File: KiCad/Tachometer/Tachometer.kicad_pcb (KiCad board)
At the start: 2 copper layers, 118.6 x 100 mm, 24 parts, among them J1 PJ301M-12, J2 Conn_01x15_MountingPin, J3 Conn_01x15_MountingPin, Q1 2N3904, Q2 2N3904

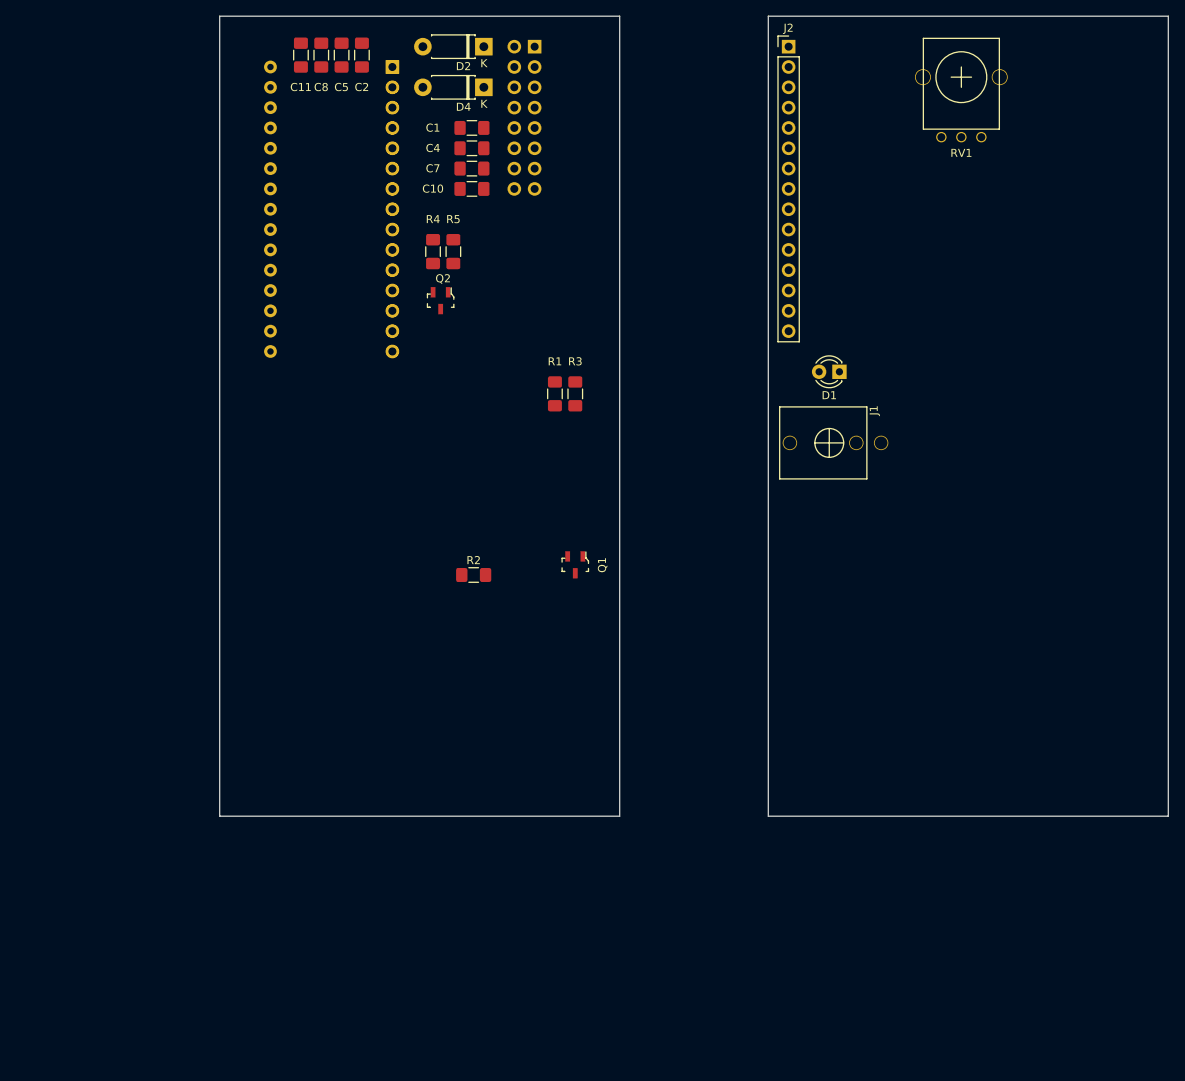
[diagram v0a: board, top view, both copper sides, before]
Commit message: ruffplaced pcb
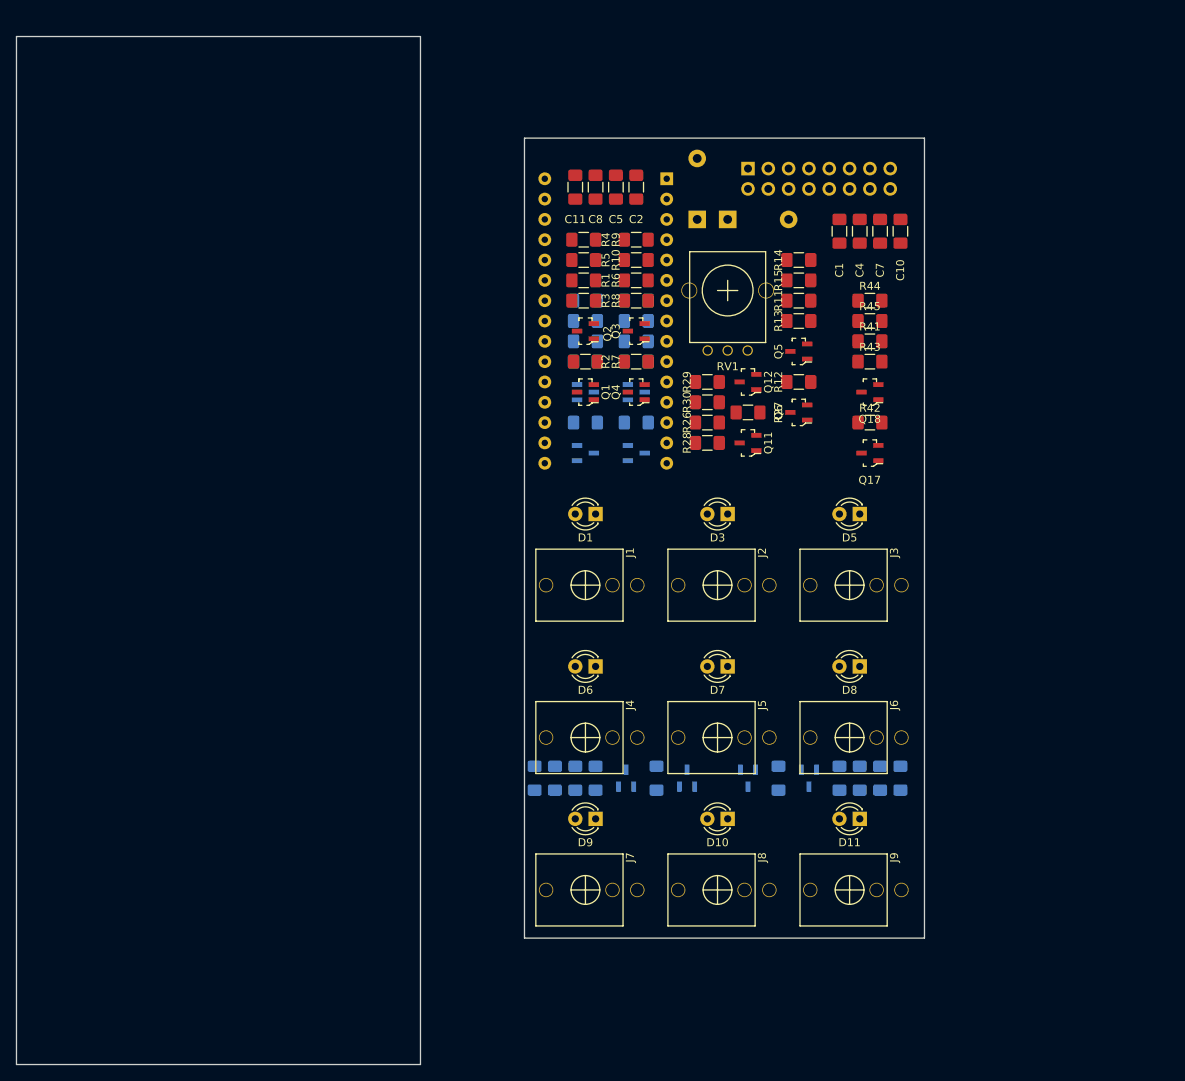
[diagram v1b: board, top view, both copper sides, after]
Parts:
- added D10: LED, LED_THT:LED_D3.0mm_FlatTop, F.Cu at (203.2, 123.2)
- added D11: LED, LED_THT:LED_D3.0mm_FlatTop, F.Cu at (219.7, 123.2)
- added D3: LED, LED_THT:LED_D3.0mm_FlatTop, F.Cu at (203.2, 85.1)
- added D5: LED, LED_THT:LED_D3.0mm_FlatTop, F.Cu at (219.7, 85.1)
- added D6: LED, LED_THT:LED_D3.0mm_FlatTop, F.Cu at (186.7, 104.1)
- added D7: LED, LED_THT:LED_D3.0mm_FlatTop, F.Cu at (203.2, 104.1)
- added D8: LED, LED_THT:LED_D3.0mm_FlatTop, F.Cu at (219.7, 104.1)
- added D9: LED, LED_THT:LED_D3.0mm_FlatTop, F.Cu at (186.7, 123.2)
- added J4: PJ301M-12, eurorack:PJ301M-12, F.Cu at (185.4, 113.0)
- added J5: PJ301M-12, eurorack:PJ301M-12, F.Cu at (201.9, 113.0)
- added J6: PJ301M-12, eurorack:PJ301M-12, F.Cu at (218.4, 113.0)
- added J7: PJ301M-12, eurorack:PJ301M-12, F.Cu at (185.4, 132.1)
- added J8: PJ301M-12, eurorack:PJ301M-12, F.Cu at (201.9, 132.1)
- added J9: PJ301M-12, eurorack:PJ301M-12, F.Cu at (218.4, 132.1)
- added Q10: 2N3904, digikey-footprints:SOT-23-3, B.Cu at (191.8, 69.8)
- added Q11: 2N3904, digikey-footprints:SOT-23-3, F.Cu at (205.7, 76.2)
- added Q12: 2N3904, digikey-footprints:SOT-23-3, F.Cu at (205.7, 68.6)
- added Q13: 2N3904, digikey-footprints:SOT-23-3, B.Cu at (198.1, 118.1)
- added Q14: 2N3904, digikey-footprints:SOT-23-3, B.Cu at (190.5, 118.1)
- added Q15: 2N3904, digikey-footprints:SOT-23-3, B.Cu at (205.7, 118.1)
- added Q16: 2N3904, digikey-footprints:SOT-23-3, B.Cu at (213.4, 118.1)
- added Q17: 2N3904, digikey-footprints:SOT-23-3, F.Cu at (221.0, 77.5)
- added Q18: 2N3904, digikey-footprints:SOT-23-3, F.Cu at (221.0, 69.8)
- added Q3: 2N3904, digikey-footprints:SOT-23-3, F.Cu at (191.8, 62.2)
- added Q4: 2N3904, digikey-footprints:SOT-23-3, F.Cu at (191.8, 69.8)
- added Q5: 2N3904, digikey-footprints:SOT-23-3, F.Cu at (212.1, 64.8)
- added Q6: 2N3904, digikey-footprints:SOT-23-3, F.Cu at (212.1, 72.4)
- added Q7: 2N3904, digikey-footprints:SOT-23-3, B.Cu at (185.4, 77.5)
- added Q8: 2N3904, digikey-footprints:SOT-23-3, B.Cu at (185.4, 69.8)
- added Q9: 2N3904, digikey-footprints:SOT-23-3, B.Cu at (191.8, 77.5)
- added R10: 200, Resistor_SMD:R_1206_3216Metric_Pad1.42x1.75mm_HandSolder, F.Cu at (191.8, 53.3)
- added R11: 1k, Resistor_SMD:R_1206_3216Metric_Pad1.42x1.75mm_HandSolder, F.Cu at (212.1, 58.4)
- added R12: 1k, Resistor_SMD:R_1206_3216Metric_Pad1.42x1.75mm_HandSolder, F.Cu at (212.1, 68.6)
- added R13: 10k, Resistor_SMD:R_1206_3216Metric_Pad1.42x1.75mm_HandSolder, F.Cu at (212.1, 61.0)
- added R14: 1k, Resistor_SMD:R_1206_3216Metric_Pad1.42x1.75mm_HandSolder, F.Cu at (212.1, 53.3)
- added R15: 200, Resistor_SMD:R_1206_3216Metric_Pad1.42x1.75mm_HandSolder, F.Cu at (212.1, 55.9)
- added R16: 1k, Resistor_SMD:R_1206_3216Metric_Pad1.42x1.75mm_HandSolder, B.Cu at (185.4, 63.5)
- added R17: 1k, Resistor_SMD:R_1206_3216Metric_Pad1.42x1.75mm_HandSolder, B.Cu at (185.4, 73.7)
- added R18: 10k, Resistor_SMD:R_1206_3216Metric_Pad1.42x1.75mm_HandSolder, B.Cu at (185.4, 66.0)
- added R19: 1k, Resistor_SMD:R_1206_3216Metric_Pad1.42x1.75mm_HandSolder, B.Cu at (185.4, 58.4)
- added R20: 200, Resistor_SMD:R_1206_3216Metric_Pad1.42x1.75mm_HandSolder, B.Cu at (185.4, 61.0)
- added R21: 1k, Resistor_SMD:R_1206_3216Metric_Pad1.42x1.75mm_HandSolder, B.Cu at (191.8, 63.5)
- added R22: 1k, Resistor_SMD:R_1206_3216Metric_Pad1.42x1.75mm_HandSolder, B.Cu at (191.8, 73.7)
- added R23: 10k, Resistor_SMD:R_1206_3216Metric_Pad1.42x1.75mm_HandSolder, B.Cu at (191.8, 66.0)
- added R24: 1k, Resistor_SMD:R_1206_3216Metric_Pad1.42x1.75mm_HandSolder, B.Cu at (191.8, 58.4)
- added R25: 200, Resistor_SMD:R_1206_3216Metric_Pad1.42x1.75mm_HandSolder, B.Cu at (191.8, 61.0)
- added R26: 1k, Resistor_SMD:R_1206_3216Metric_Pad1.42x1.75mm_HandSolder, F.Cu at (200.7, 73.7)
- added R27: 1k, Resistor_SMD:R_1206_3216Metric_Pad1.42x1.75mm_HandSolder, F.Cu at (205.7, 72.4)
- added R28: 10k, Resistor_SMD:R_1206_3216Metric_Pad1.42x1.75mm_HandSolder, F.Cu at (200.7, 76.2)
- added R29: 1k, Resistor_SMD:R_1206_3216Metric_Pad1.42x1.75mm_HandSolder, F.Cu at (200.7, 68.6)
- added R30: 200, Resistor_SMD:R_1206_3216Metric_Pad1.42x1.75mm_HandSolder, F.Cu at (200.7, 71.1)
- added R31: 1k, Resistor_SMD:R_1206_3216Metric_Pad1.42x1.75mm_HandSolder, B.Cu at (184.2, 118.1)
- added R32: 1k, Resistor_SMD:R_1206_3216Metric_Pad1.42x1.75mm_HandSolder, B.Cu at (194.3, 118.1)
- added R33: 10k, Resistor_SMD:R_1206_3216Metric_Pad1.42x1.75mm_HandSolder, B.Cu at (186.7, 118.1)
- added R34: 1k, Resistor_SMD:R_1206_3216Metric_Pad1.42x1.75mm_HandSolder, B.Cu at (179.1, 118.1)
- added R35: 200, Resistor_SMD:R_1206_3216Metric_Pad1.42x1.75mm_HandSolder, B.Cu at (181.6, 118.1)
- added R36: 1k, Resistor_SMD:R_1206_3216Metric_Pad1.42x1.75mm_HandSolder, B.Cu at (219.7, 118.1)
- added R37: 1k, Resistor_SMD:R_1206_3216Metric_Pad1.42x1.75mm_HandSolder, B.Cu at (209.6, 118.1)
- added R38: 10k, Resistor_SMD:R_1206_3216Metric_Pad1.42x1.75mm_HandSolder, B.Cu at (217.2, 118.1)
- added R39: 1k, Resistor_SMD:R_1206_3216Metric_Pad1.42x1.75mm_HandSolder, B.Cu at (224.8, 118.1)
- added R40: 200, Resistor_SMD:R_1206_3216Metric_Pad1.42x1.75mm_HandSolder, B.Cu at (222.2, 118.1)
- added R41: 1k, Resistor_SMD:R_1206_3216Metric_Pad1.42x1.75mm_HandSolder, F.Cu at (221.0, 63.5)
- added R42: 1k, Resistor_SMD:R_1206_3216Metric_Pad1.42x1.75mm_HandSolder, F.Cu at (221.0, 73.7)
- added R43: 10k, Resistor_SMD:R_1206_3216Metric_Pad1.42x1.75mm_HandSolder, F.Cu at (221.0, 66.0)
- added R44: 1k, Resistor_SMD:R_1206_3216Metric_Pad1.42x1.75mm_HandSolder, F.Cu at (221.0, 58.4)
- added R45: 200, Resistor_SMD:R_1206_3216Metric_Pad1.42x1.75mm_HandSolder, F.Cu at (221.0, 61.0)
- added R6: 1k, Resistor_SMD:R_1206_3216Metric_Pad1.42x1.75mm_HandSolder, F.Cu at (191.8, 55.9)
- added R7: 1k, Resistor_SMD:R_1206_3216Metric_Pad1.42x1.75mm_HandSolder, F.Cu at (191.8, 66.0)
- added R8: 10k, Resistor_SMD:R_1206_3216Metric_Pad1.42x1.75mm_HandSolder, F.Cu at (191.8, 58.4)
- added R9: 1k, Resistor_SMD:R_1206_3216Metric_Pad1.42x1.75mm_HandSolder, F.Cu at (191.8, 50.8)
- D2, D4: moved to B.Cu
- J2: value Conn_01x15_MountingPin -> PJ301M-12; footprint Connector_PinHeader_2.54mm:PinHeader_1x15_P2.54mm_Vertical -> eurorack:PJ301M-12
- J3: value Conn_01x15_MountingPin -> PJ301M-12; footprint Connector_PinHeader_2.54mm:PinHeader_1x15_P2.54mm_Vertical -> eurorack:PJ301M-12; moved to F.Cu
- moved J3 86.4 mm to (218.4, 94.0), turned to 90 degrees
- moved J2 67.9 mm to (201.9, 94.0), turned to 90 degrees
- moved C10 53.8 mm to (224.8, 49.7), turned to 90 degrees
- moved C7 51.6 mm to (222.2, 49.7), turned to 90 degrees
- moved C4 49.6 mm to (219.7, 49.7), turned to 90 degrees
- moved C1 47.7 mm to (217.2, 49.7), turned to 90 degrees
- moved RV1 39.6 mm to (203.2, 57.1)
- moved C2 38.1 mm to (191.8, 44.2)
- moved C11 38.1 mm to (184.2, 44.2)
- moved C5 38.1 mm to (189.2, 44.2)
- moved C8 38.1 mm to (186.7, 44.2)
- moved A1 37.0 mm to (195.6, 43.2)
- moved J1 35.3 mm to (185.4, 94.0)
- moved D1 35.3 mm to (186.7, 85.1)
- moved D4 34.7 mm to (203.2, 48.3), turned to 0 degrees
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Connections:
- A1 pad 10: Net-(A1-Pad10) -> Tr6
- A1 pad 11: Net-(A1-Pad11) -> Tr7
- A1 pad 12: Net-(A1-Pad12) -> Tr8
- A1 pad 13: Net-(A1-Pad13) -> Tr9
- A1 pad 5: Net-(A1-Pad5) -> Tr1
- A1 pad 6: Net-(A1-Pad6) -> Tr2
- A1 pad 7: Net-(A1-Pad7) -> Tr3
- A1 pad 8: Net-(A1-Pad8) -> Tr4
- A1 pad 9: Net-(A1-Pad9) -> Tr5
- J2 pad 1: Net-(J2-Pad1) -> GND
- J2 pad 2: Net-(J2-Pad2) -> GND
- J3 pad 1: Net-(J3-Pad1) -> GND
- J3 pad 2: Net-(J3-Pad2) -> GND
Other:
- board size 118.6 x 100 mm -> 113.5 x 128.5 mm

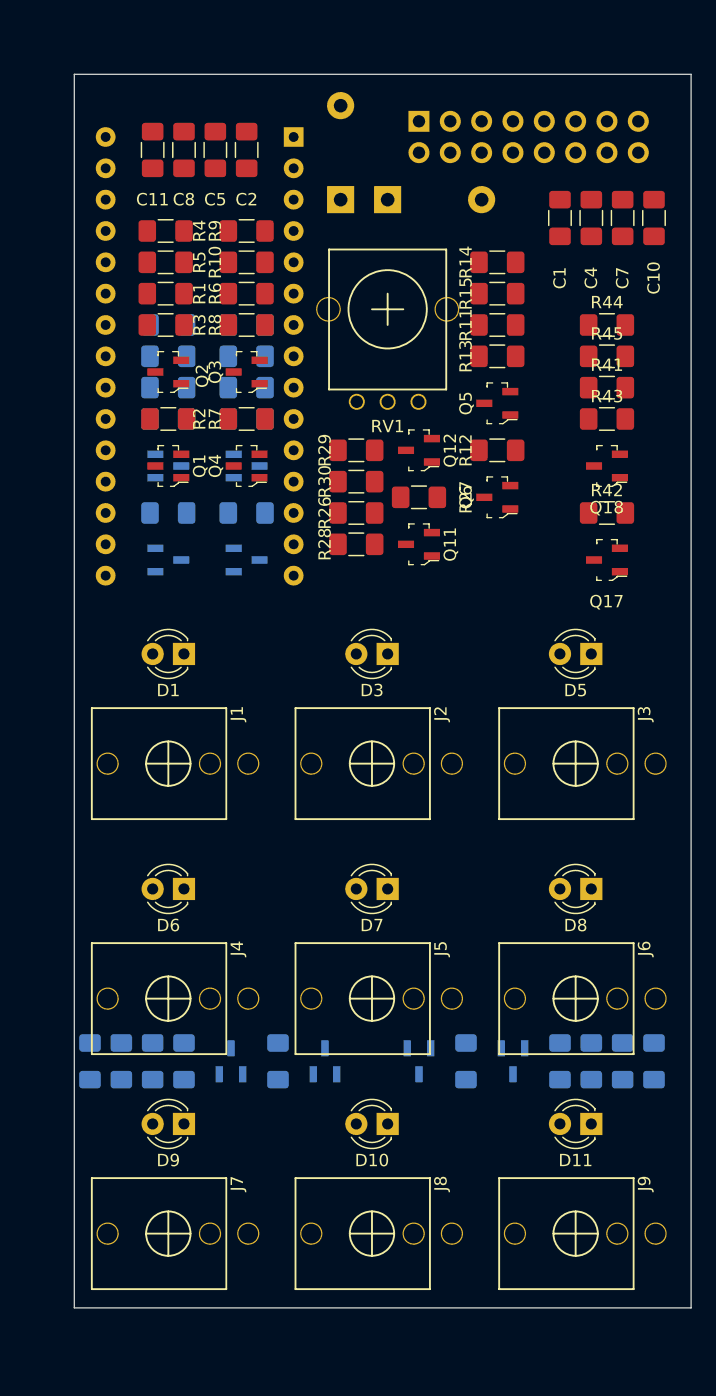
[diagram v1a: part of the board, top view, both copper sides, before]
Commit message: workworkwork
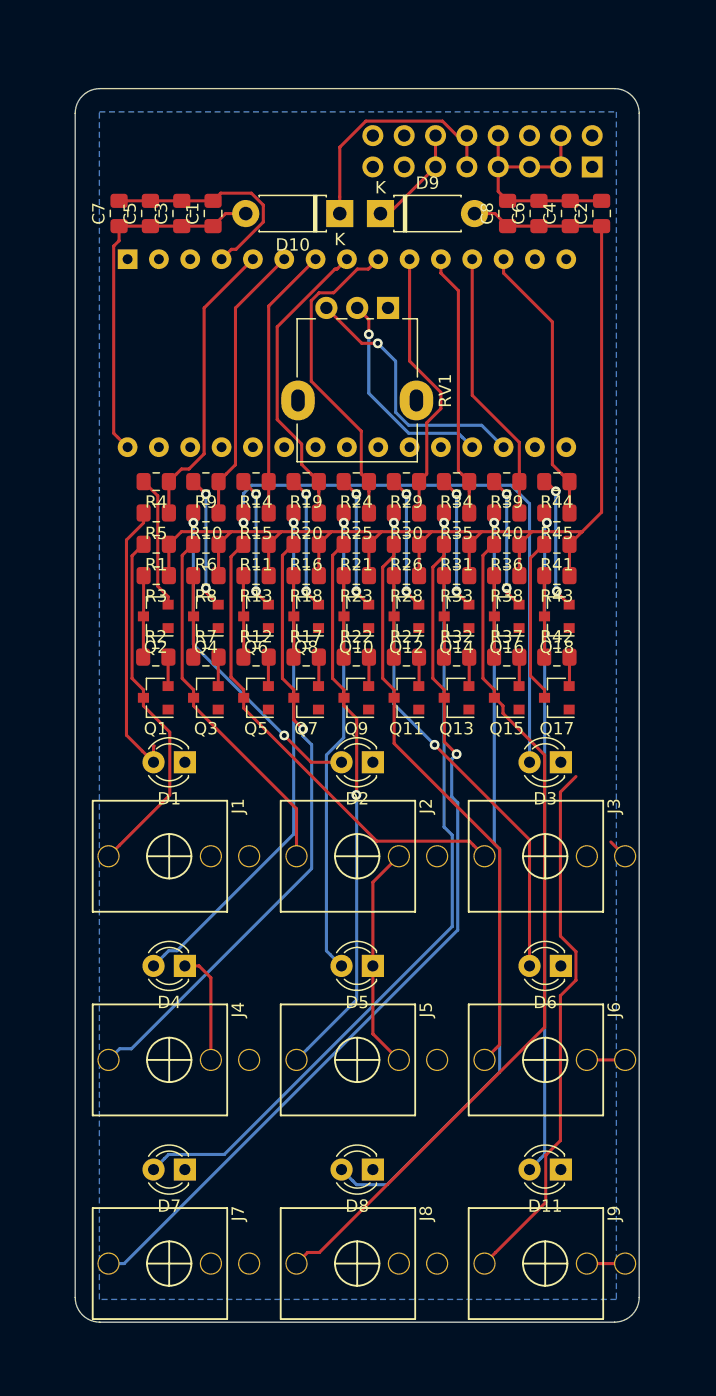
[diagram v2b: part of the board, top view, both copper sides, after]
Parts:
- removed the D2 at (199.4, 48.3)
- added D10: 1N4006, Diode_THT:D_DO-41_SOD81_P7.62mm_Horizontal, F.Cu at (199.3, 49.4)
- C1: renamed from C11; footprint Capacitor_SMD:C_1206_3216Metric_Pad1.42x1.75mm_HandSolder -> Capacitor_SMD:C_0805_2012Metric_Pad1.15x1.40mm_HandSolder
- C2: renamed from C10; footprint Capacitor_SMD:C_1206_3216Metric_Pad1.42x1.75mm_HandSolder -> Capacitor_SMD:C_0805_2012Metric_Pad1.15x1.40mm_HandSolder
- C3: renamed from C8; footprint Capacitor_SMD:C_1206_3216Metric_Pad1.42x1.75mm_HandSolder -> Capacitor_SMD:C_0805_2012Metric_Pad1.15x1.40mm_HandSolder
- C4: renamed from C7; footprint Capacitor_SMD:C_1206_3216Metric_Pad1.42x1.75mm_HandSolder -> Capacitor_SMD:C_0805_2012Metric_Pad1.15x1.40mm_HandSolder
- C5: footprint Capacitor_SMD:C_1206_3216Metric_Pad1.42x1.75mm_HandSolder -> Capacitor_SMD:C_0805_2012Metric_Pad1.15x1.40mm_HandSolder
- C6: renamed from C4; footprint Capacitor_SMD:C_1206_3216Metric_Pad1.42x1.75mm_HandSolder -> Capacitor_SMD:C_0805_2012Metric_Pad1.15x1.40mm_HandSolder
- C7: renamed from C2; footprint Capacitor_SMD:C_1206_3216Metric_Pad1.42x1.75mm_HandSolder -> Capacitor_SMD:C_0805_2012Metric_Pad1.15x1.40mm_HandSolder
- C8: renamed from C1; footprint Capacitor_SMD:C_1206_3216Metric_Pad1.42x1.75mm_HandSolder -> Capacitor_SMD:C_0805_2012Metric_Pad1.15x1.40mm_HandSolder
- D9: renamed from D4; moved to F.Cu
- Q1, Q11, Q12, Q17, Q18, Q2, Q3, Q4, Q5, Q6: footprint digikey-footprints:SOT-23-3 -> Package_TO_SOT_SMD:SOT-23
- Q10, Q13, Q14, Q15, Q16, Q7, Q8, Q9: footprint digikey-footprints:SOT-23-3 -> Package_TO_SOT_SMD:SOT-23; moved to F.Cu
- R1, R10, R11, R12, R13, R14, R15, R2, R26, R27, R28, R29, R3, R30, R4, R41, R42, R43, R44, R45, R5, R6, R7, R8, R9: footprint Resistor_SMD:R_1206_3216Metric_Pad1.42x1.75mm_HandSolder -> Resistor_SMD:R_0805_2012Metric_Pad1.15x1.40mm_HandSolder
- R16, R17, R18, R19, R20, R21, R22, R23, R24, R25, R31, R32, R33, R34, R35, R36, R37, R38, R39, R40: footprint Resistor_SMD:R_1206_3216Metric_Pad1.42x1.75mm_HandSolder -> Resistor_SMD:R_0805_2012Metric_Pad1.15x1.40mm_HandSolder; moved to F.Cu
- RV1: footprint eurorack:Alpha9mmPot -> Potentiometer_THT:Potentiometer_Alpha_RD901F-40-00D_Single_Vertical
- moved R34 55.6 mm to (208.8, 71.1), turned to 180 degrees
- moved R35 52.1 mm to (208.8, 73.7), turned to 180 degrees
- moved R31 48.6 mm to (208.8, 76.2), turned to 180 degrees
- moved R39 48.5 mm to (212.9, 71.1), turned to 180 degrees
- moved R40 45.4 mm to (212.9, 73.7), turned to 180 degrees
- moved R33 45.1 mm to (208.8, 78.7), turned to 180 degrees
- moved R36 42.5 mm to (212.9, 76.2), turned to 180 degrees
- moved Q14 40.4 mm to (208.8, 82.0), turned to 180 degrees
- moved R38 39.6 mm to (212.9, 78.7), turned to 180 degrees
- moved Q16 36.1 mm to (212.9, 82.0), turned to 180 degrees
- moved R32 35.8 mm to (208.8, 85.3), turned to 0 degrees
- moved R37 32.9 mm to (212.9, 85.3), turned to 0 degrees
- moved Q13 31.3 mm to (208.8, 88.6), turned to 180 degrees
- moved Q5 30.9 mm to (192.5, 88.6)
- moved Q15 30.3 mm to (212.9, 88.6), turned to 180 degrees
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- renumbered D3 to D2, D5 to D3, D6 to D4, D7 to D5, D8 to D6, D9 to D7, D10 to D8
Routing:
- net 5V: track 0.00 -> 104.5 mm
- net GND: track 0.00 -> 74.5 mm
- net Net-(J7-Pad3): track 0.00 -> 72.3 mm, vias 0 -> 1
- net Net-(J8-Pad3): track 0.00 -> 69.7 mm
- net Net-(D7-Pad2): track 0.00 -> 66.2 mm, vias 0 -> 1
- net Net-(D8-Pad2): track 0.00 -> 62.6 mm, vias 0 -> 1
- net Net-(J9-Pad3): track 0.00 -> 57.0 mm
- net Net-(D11-Pad2): track 0.00 -> 53.9 mm, vias 0 -> 1
- net Net-(J4-Pad3): track 0.00 -> 50.5 mm, vias 0 -> 1
- net Net-(D3-Pad2): track 0.00 -> 48.5 mm, vias 0 -> 1
- net Net-(J6-Pad3): track 0.00 -> 46.6 mm
- net Net-(J5-Pad3): track 0.00 -> 45.0 mm, vias 0 -> 1
- net Net-(D4-Pad2): track 0.00 -> 42.1 mm, vias 0 -> 1
- net Net-(D6-Pad2): track 0.00 -> 41.3 mm, vias 0 -> 2
- net Net-(J3-Pad3): track 0.00 -> 38.6 mm
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- added copper zone on B.Cu, net GND
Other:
- board size 113.5 x 128.5 mm -> 109.3 x 128.5 mm
